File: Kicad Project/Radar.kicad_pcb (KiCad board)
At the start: 2 copper layers, 100 x 100 mm, 90 parts, among them J1 Conn_01x02, J2 Conn_01x02, J3 Conn_01x02, J4 Conn_01x02, J5 Conn_01x02, J6 Conn_01x02, J7 Conn_01x02, U1 GALI-1+, U10 GALI-2+, U11 BandpassFilter, U12 ufl, U13 Antenna111, U14 Antenna111, U15 ufl, U16 TC1185, U2 MCA1-85L+, U3 BandpassFilter, U4 LMV751, U5 AP1117-50, U6 GALI-2+, U7 RMK-3-93+, U8 GALI-2+, U9 LEE-39+

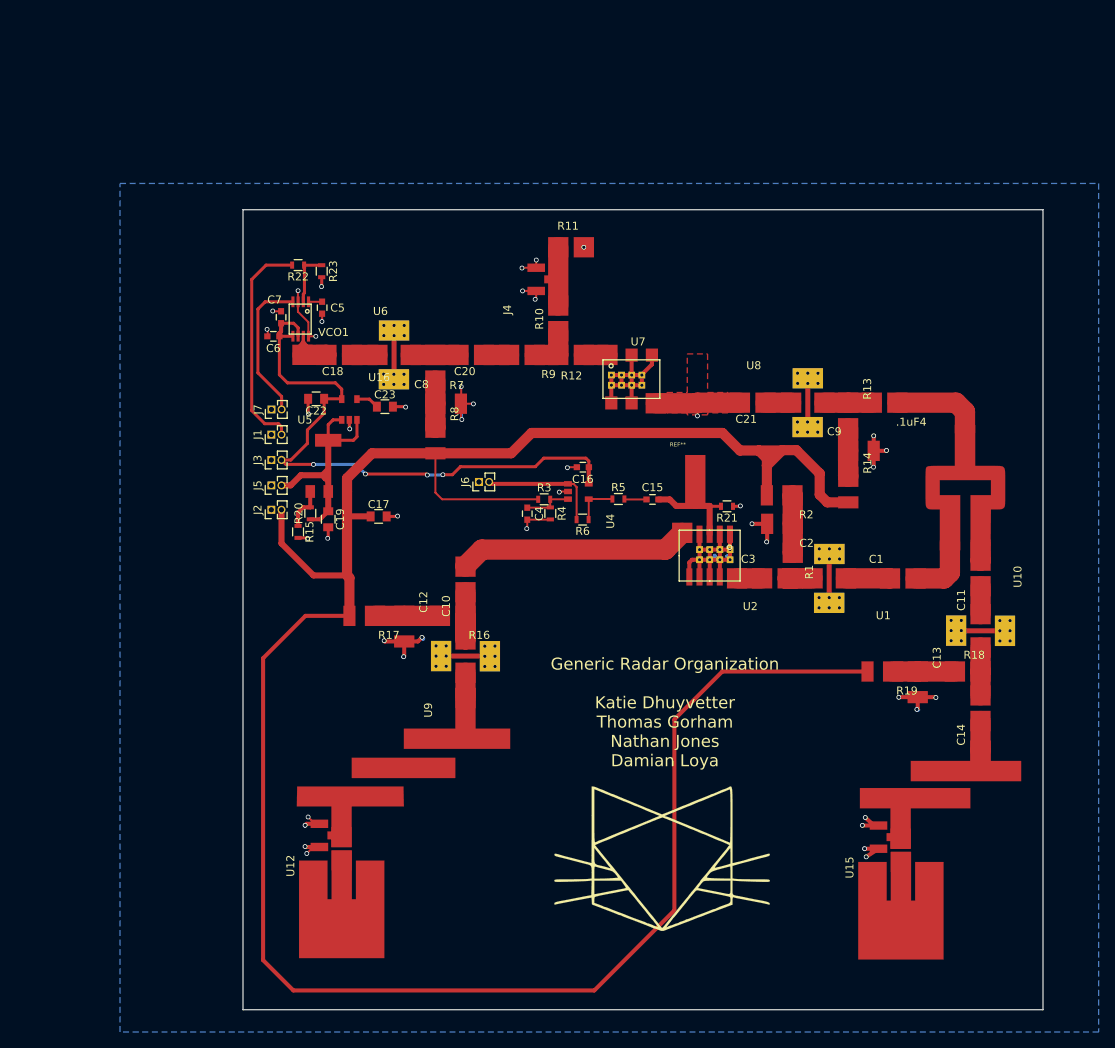
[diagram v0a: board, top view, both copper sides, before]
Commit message: updated gerbers
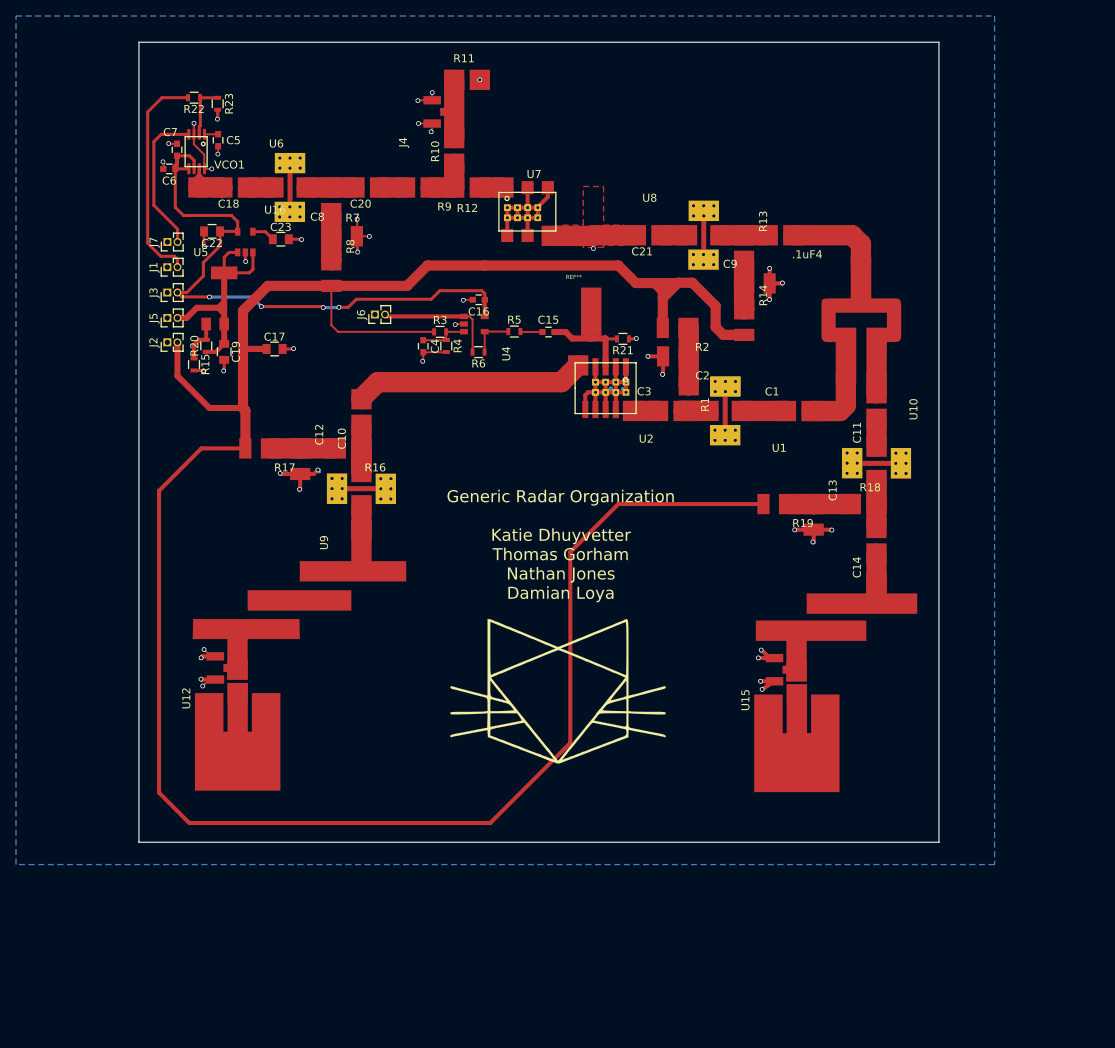
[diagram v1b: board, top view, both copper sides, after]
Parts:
- moved .1uF4 24.6 mm to (161.9, 78.3)
- moved ? 24.6 mm to (141.0, 99.2)
- moved ? 24.6 mm to (128.7, 77.4)
- moved ? 24.6 mm to (128.7, 76.1)
- moved C21 24.6 mm to (145.4, 78.3)
- moved R14 24.6 mm to (155.8, 90.1)
- moved ? 24.6 mm to (141.0, 97.9)
- moved ? 24.6 mm to (127.4, 77.4)
- moved ? 24.6 mm to (127.4, 76.1)
- moved C1 24.6 mm to (163.5, 102.8)
- moved C10 24.6 mm to (110.5, 102.0)
- moved C11 24.6 mm to (174.9, 101.2)
- moved C16 24.6 mm to (123.9, 87.6)
- moved C5 24.6 mm to (91.3, 67.7)
- moved C8 24.6 mm to (106.7, 80.9)
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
